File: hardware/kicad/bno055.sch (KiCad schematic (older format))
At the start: 7 parts, among them U4 BNO055

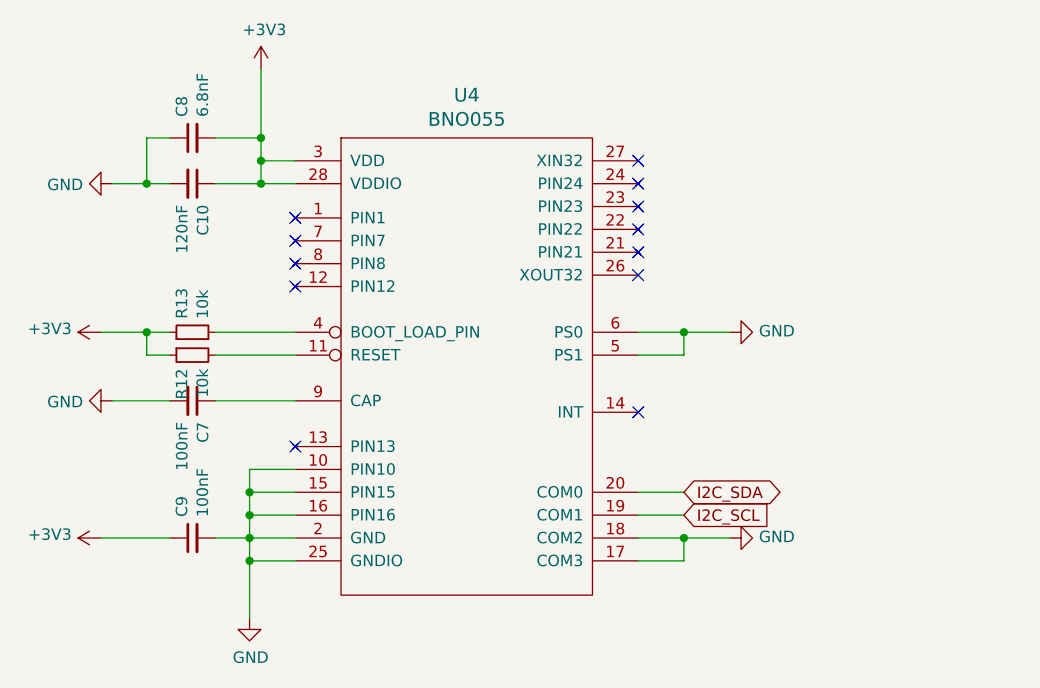
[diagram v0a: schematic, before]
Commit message: finished layout
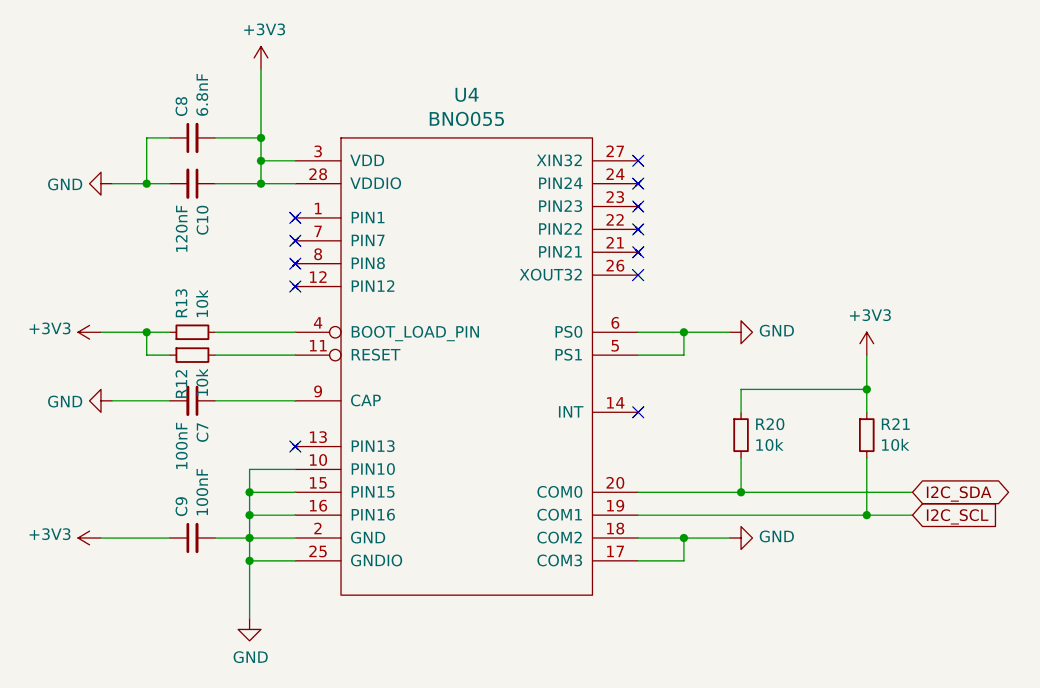
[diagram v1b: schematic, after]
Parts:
- added R20, R21: 10k, resistors:R_0603, symbol devices:R_0603
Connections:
- net +3V3: now also R20.1, R21.1
- net I2C_SCL: now also R21.2
- net I2C_SDA: now also R20.2
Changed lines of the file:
@@
 Wire Wire Line
 	3350 4300 3050 4300
-Text GLabel 5600 4100 2    50   BiDi ~ 0
+Text GLabel 6600 4100 2    50   BiDi ~ 0
 I2C_SDA
-Text GLabel 5600 4200 2    50   Input ~ 0
+Text GLabel 6600 4200 2    50   Input ~ 0
 I2C_SCL
 Wire Wire Line
-	5600 4100 5400 4100
+	5400 4100 5850 4100
 Wire Wire Line
-	5400 4200 5600 4200
+	5400 4200 6400 4200
+$Comp
+L devices:R_0603 R20
+U 1 1 5E97804D
+P 5850 3850
+F 0 "R20" H 5909 3896 50  0000 L CNN
+F 1 "10k" H 5909 3805 50  0000 L CNN
+F 2 "resistors:R_0603" H 5850 3700 50  0001 C CNN
+F 3 "" H 5850 3850 50  0000 C CNN
+	1    5850 3850
+	1    0    0    -1
+$EndComp
+$Comp
+L devices:R_0603 R21
+U 1 1 5E9781BC
+P 6400 3850
+F 0 "R21" H 6459 3896 50  0000 L CNN
+F 1 "10k" H 6459 3805 50  0000 L CNN
+F 2 "resistors:R_0603" H 6400 3700 50  0001 C CNN
+F 3 "" H 6400 3850 50  0000 C CNN
+	1    6400 3850
+	1    0    0    -1
+$EndComp
+Wire Wire Line
+	5850 4100 5850 3950
+Connection ~ 5850 4100
+Wire Wire Line
+	5850 4100 6600 4100
+Wire Wire Line
+	6400 3950 6400 4200
+Connection ~ 6400 4200
+Wire Wire Line
+	6400 4200 6600 4200
+Wire Wire Line
+	5850 3750 5850 3650
+Wire Wire Line
+	5850 3650 6400 3650
+Wire Wire Line
+	6400 3650 6400 3750
+$Comp
+L power-supply:+3V3 #PWR?
+U 1 1 5E97B2A1
+P 6400 3500
+F 0 "#PWR?" H 6400 3350 50  0001 C CNN
+F 1 "+3V3" H 6415 3673 50  0000 C CNN
+F 2 "" H 6400 3500 50  0000 C CNN
+F 3 "" H 6400 3500 50  0000 C CNN
+	1    6400 3500
+	1    0    0    -1
+$EndComp
+Wire Wire Line
+	6400 3500 6400 3650
+Connection ~ 6400 3650
 $EndSCHEMATC
